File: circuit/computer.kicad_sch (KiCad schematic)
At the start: 20 parts, among them J1 Mega2560 Left, J11 IO3, J12 Ext. Clock, J2 IO2, J3 USB-C Power, J4 Mega2560 Right, J7 IO1, SW2 Debug, U2 Z80CPU, U3 AS6C4008-55PCN

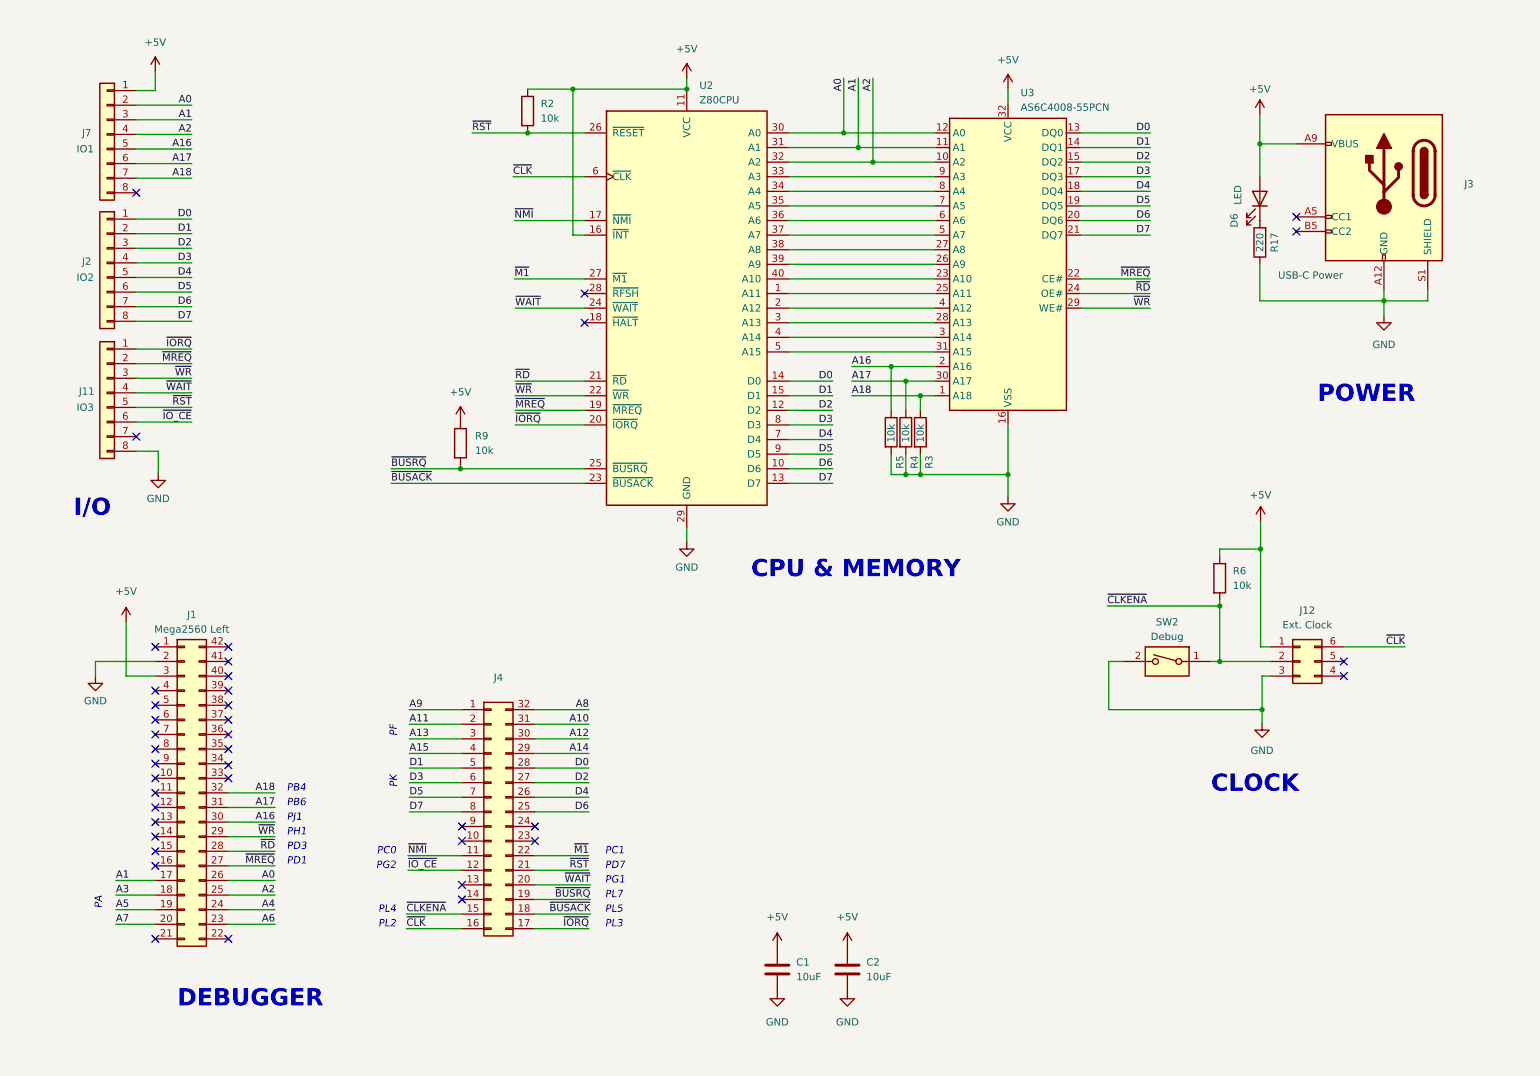
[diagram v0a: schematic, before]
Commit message: .
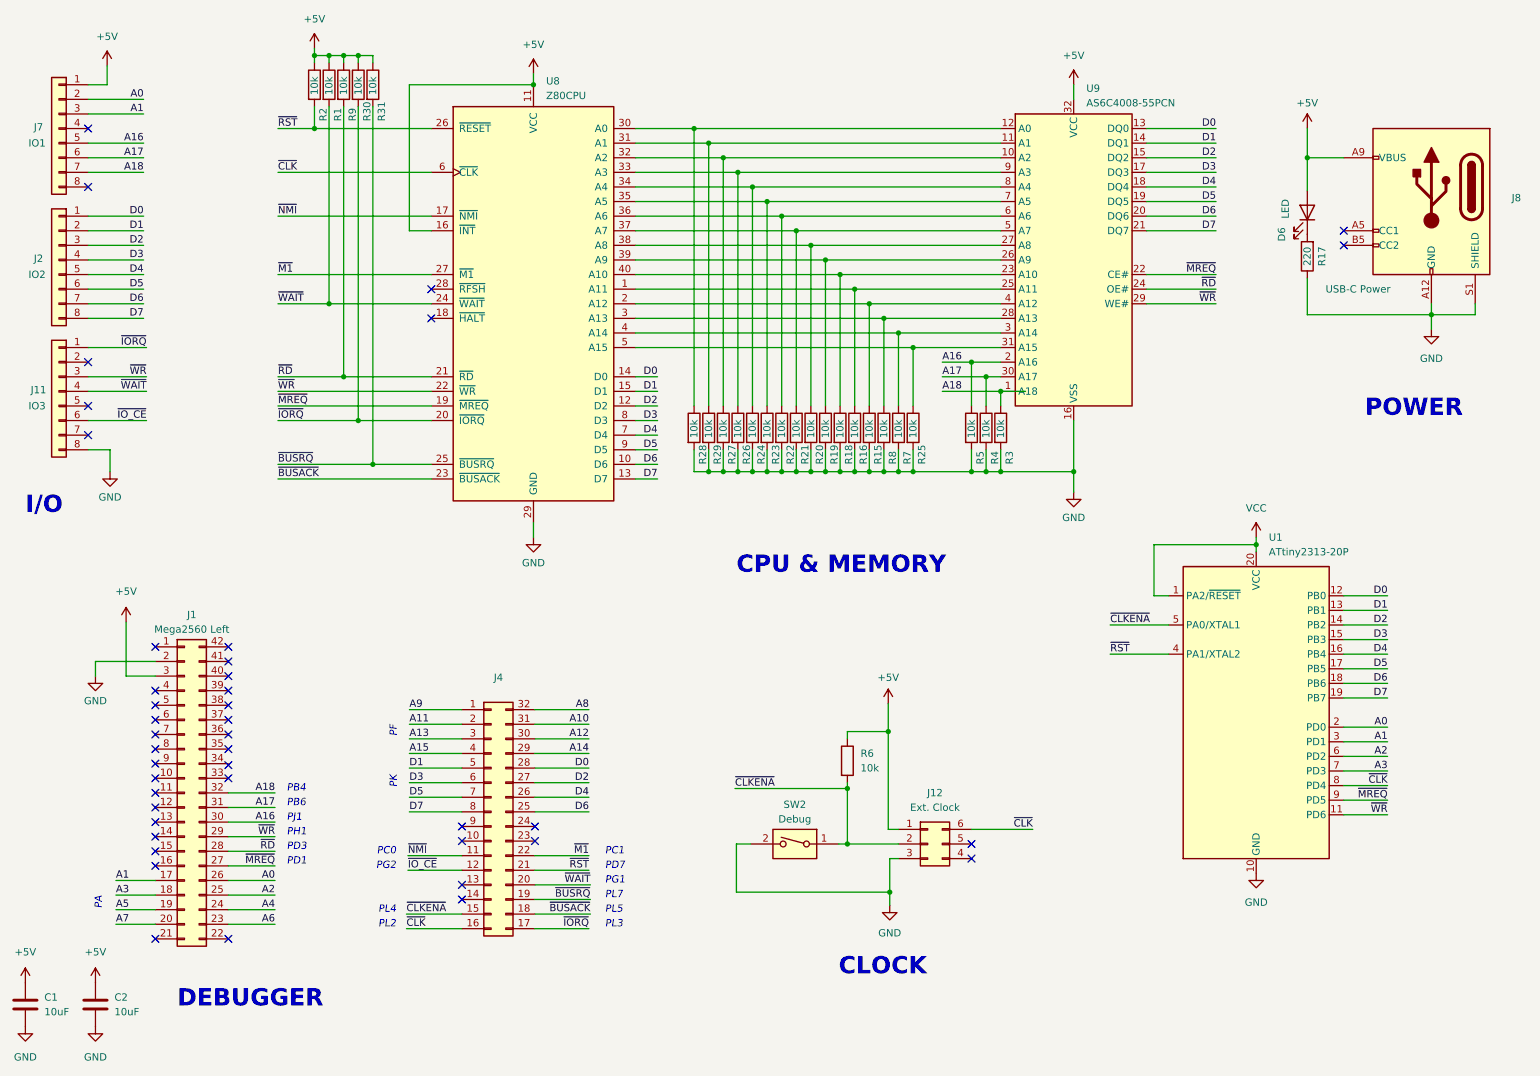
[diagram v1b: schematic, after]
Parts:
- added R1, R15, R16, R18, R19, R20, R21, R22, R23, R24, R25, R26, R27, R28, R29, R30, R31, R7, R8: 10k, symbol Device:R
- added U1: ATtiny2313-20P, Package_DIP:DIP-20_W7.62mm, symbol MCU_Microchip_ATtiny:ATtiny2313-20P
- renumbered J3 to J8, U2 to U8, U3 to U9
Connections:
- net +5V: now also R1.1, R30.1, R31.1
- net A0: now also U1.2 (PD0); no longer U8.30 (A0), U9.12 (A0)
- net A1: now also U1.3 (PD1); no longer U8.31 (A1), U9.11 (A1)
- net A2: now also U1.6 (PD2); no longer J7.4 (Pin_4), U8.32 (A2), U9.10 (A2)
- net A3: now also U1.7 (PD3)
- net D0: now also U1.12 (PB0)
- net D1: now also U1.13 (PB1)
- net D2: now also U1.14 (PB2)
- net D3: now also U1.15 (PB3)
- net D4: now also U1.16 (PB4)
- net D5: now also U1.17 (PB5)
- net D6: now also U1.18 (PB6)
- net D7: now also U1.19 (PB7)
- net GND: now also R15.2, R16.2, R18.2, R19.2, R20.2, R21.2, R22.2, R23.2, R24.2, R25.2, R26.2, R27.2, R28.2, R29.2, R7.2, R8.2, U1.10 (GND)
- net ~{BUSRQ}: now also R31.2; no longer R9.2
- net ~{CLKENA}: now also U1.5 (PA0/XTAL1)
- net ~{CLK}: now also U1.8 (PD4)
- net ~{IORQ}: now also R30.2
- net ~{MREQ}: now also U1.9 (PD5); no longer J11.2 (Pin_2)
- net ~{RD}: now also R9.2
- net ~{RST}: now also U1.4 (PA1/XTAL2); no longer J11.5 (Pin_5)
- net ~{WAIT}: now also R1.2
- net ~{WR}: now also U1.11 (PD6)
- net at U8.1 (A11), U9.25 (A11): now also R16.1
- net at U8.2 (A12), U9.4 (A12): now also R15.1
- net at U8.3 (A13), U9.28 (A13): now also R8.1
- net at U8.33 (A3), U9.9 (A3): now also R26.1
- net at U8.34 (A4), U9.8 (A4): now also R24.1
- net at U8.35 (A5), U9.7 (A5): now also R23.1
- net at U8.36 (A6), U9.6 (A6): now also R22.1
- net at U8.37 (A7), U9.5 (A7): now also R21.1
- net at U8.38 (A8), U9.27 (A8): now also R20.1
- net at U8.39 (A9), U9.26 (A9): now also R19.1
- net at U8.4 (A14), U9.3 (A14): now also R7.1
- net at U8.40 (A10), U9.23 (A10): now also R18.1
- net at U8.5 (A15), U9.31 (A15): now also R25.1
- new net: R28.1, U8.30 (A0), U9.12 (A0)
- new net: R29.1, U8.31 (A1), U9.11 (A1)
- new net: R27.1, U8.32 (A2), U9.10 (A2)
- new net VCC: U1.1 (PA2/~{RESET}), U1.20 (VCC)
- no-connect marks 40 -> 43
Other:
- moved on the sheet: C1, C2, D6, J11, J12, J2, J7, J8, R17, R3, R4, R5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
